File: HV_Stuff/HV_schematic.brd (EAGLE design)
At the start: 101.3 x 62.2 mm, 9 parts

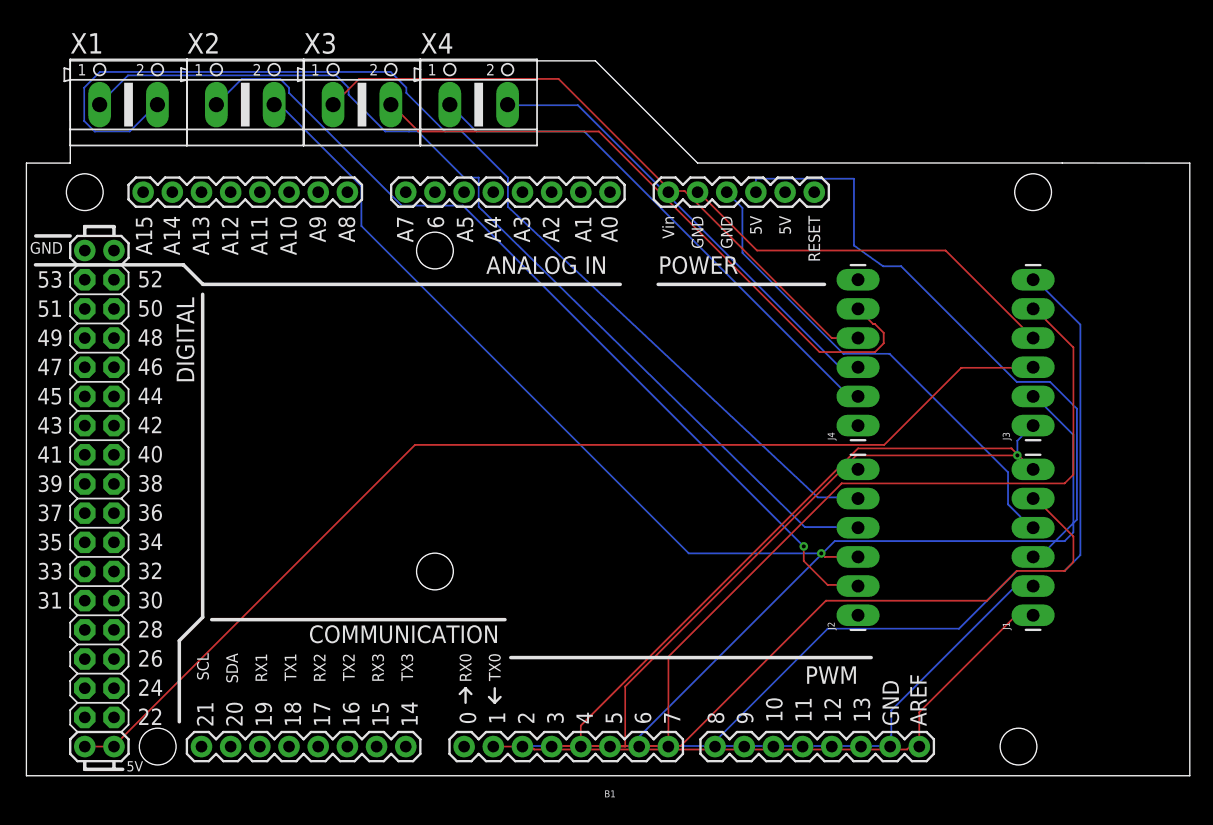
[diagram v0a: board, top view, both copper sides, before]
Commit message: Made it, it's gorgeous. It looks very pretty
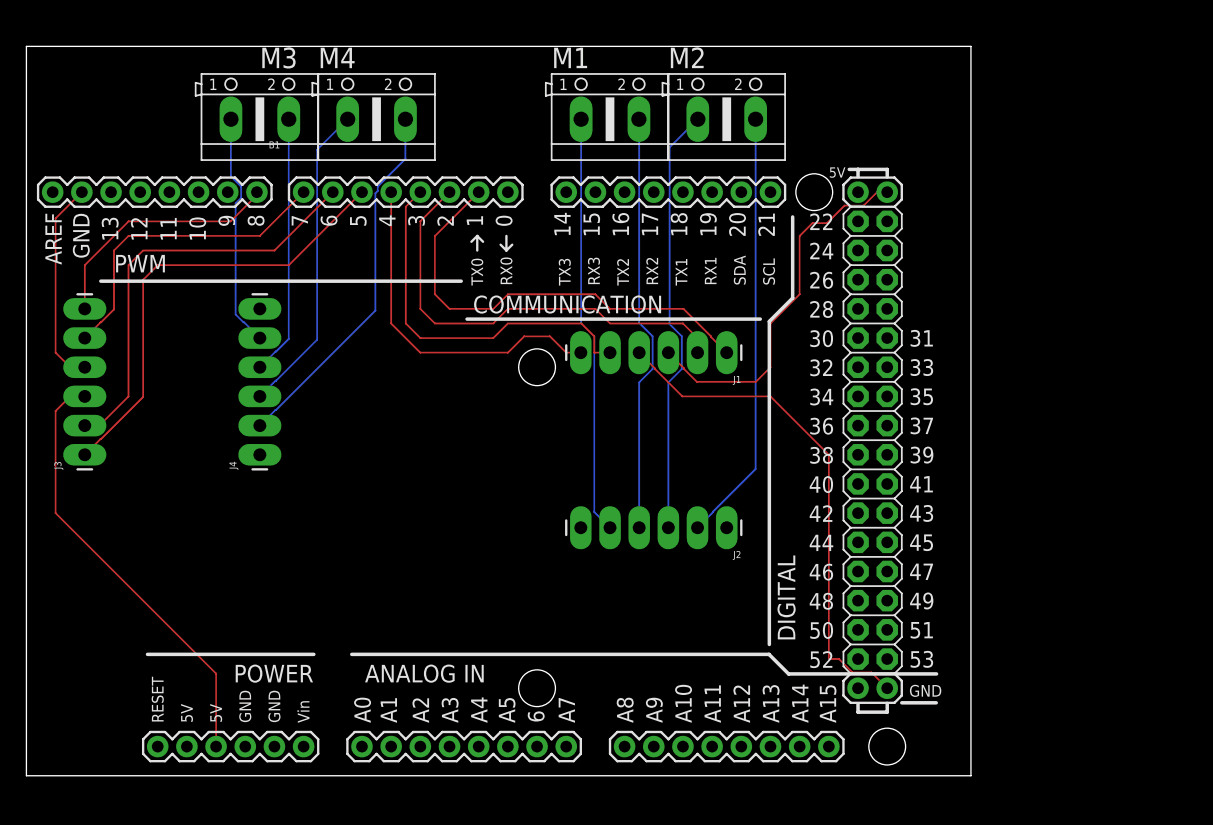
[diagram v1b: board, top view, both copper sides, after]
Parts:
- removed X1, X2, X3, X4: (no value), con-ptr500:AK500/2
- added M1, M2, M3, M4: (no value), con-ptr500:AK500/2
- B1: device SparkFun-Boards:ARDUINO_MEGA -> Will Library:ARDUINO_MEGA
- moved J3 82.6 mm to (5.08, 27.9)
- moved J4 52.1 mm to (20.3, 27.9)
- moved J1 35.1 mm to (61.0, 36.8), turned to 180 degrees
- moved B1 24.1 mm to (27.9, 26.7), turned to 0 degrees
- moved J2 13.7 mm to (61.0, 21.6), turned to 180 degrees
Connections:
- net IN1 renamed IN1_1
- net IN2 renamed IN2_1
- net IN3 renamed IN3_1
- net IN4 renamed IN4_1
- removed net GND: B1.GND@0, J1.4
- removed net GND2: B1.GND@1, J3.4
- removed net OUT1: J2.5, X1.2
- removed net OUT2: J2.4, X1.1
- removed net OUT3: J2.3, X2.2
- removed net OUT4: J2.2, X2.1
- removed net VCC: B1.5V@0, J1.3
- removed net VCC2: B1.5V@1, B1.5V@2, J3.3
- new net 5V_1: B1.5V@2, J1.3
- new net 5V_2: B1.5V@0, J3.3
- new net GND_1: B1.GND@3, J1.4
- new net GND_2: B1.GND@4, J3.4
- new net N$1: J2.3, M2.1
- new net OUT1_1: J2.5, M1.1
- new net OUT2_1: J2.4, M1.2
- new net OUT4_1: J2.2, M2.2
- net OUT1_2: now also M3.1; no longer X3.2
- net OUT2_2: now also M3.2; no longer X3.1
- net OUT3_2: now also M4.1; no longer X4.2
- net OUT4_2: now also M4.2; no longer X4.1
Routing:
- net VCC2: track 96.3 -> 0.00 mm
- net OUT1: track 95.2 -> 0.00 mm
- net OUT2: track 85.1 -> 0.00 mm
- net OUT4: track 76.1 -> 0.00 mm, vias 1 -> 0
- net OUT3: track 69.2 -> 0.00 mm, vias 1 -> 0
- net VCC: track 55.4 -> 0.00 mm
- net GND_1: track 0.00 -> 44.1 mm
- net IN4_2: track 64.9 -> 21.6 mm
- net GND: track 42.8 -> 0.00 mm
- net IN3_2: track 65.6 -> 27.3 mm
- net 5V_2: track 0.00 -> 38.1 mm
- net OUT4_1: track 0.00 -> 37.7 mm
- net N$1: track 0.00 -> 37.5 mm
- net OUT1_1: track 0.00 -> 36.6 mm
- net OUT2_1: track 0.00 -> 36.5 mm
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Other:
- board size 101.3 x 62.2 mm -> 82.2 x 63.5 mm
